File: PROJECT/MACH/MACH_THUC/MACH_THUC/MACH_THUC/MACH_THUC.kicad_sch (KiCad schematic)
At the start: 32 parts, among them Q1 2SB688, U1 LM7805_TO220

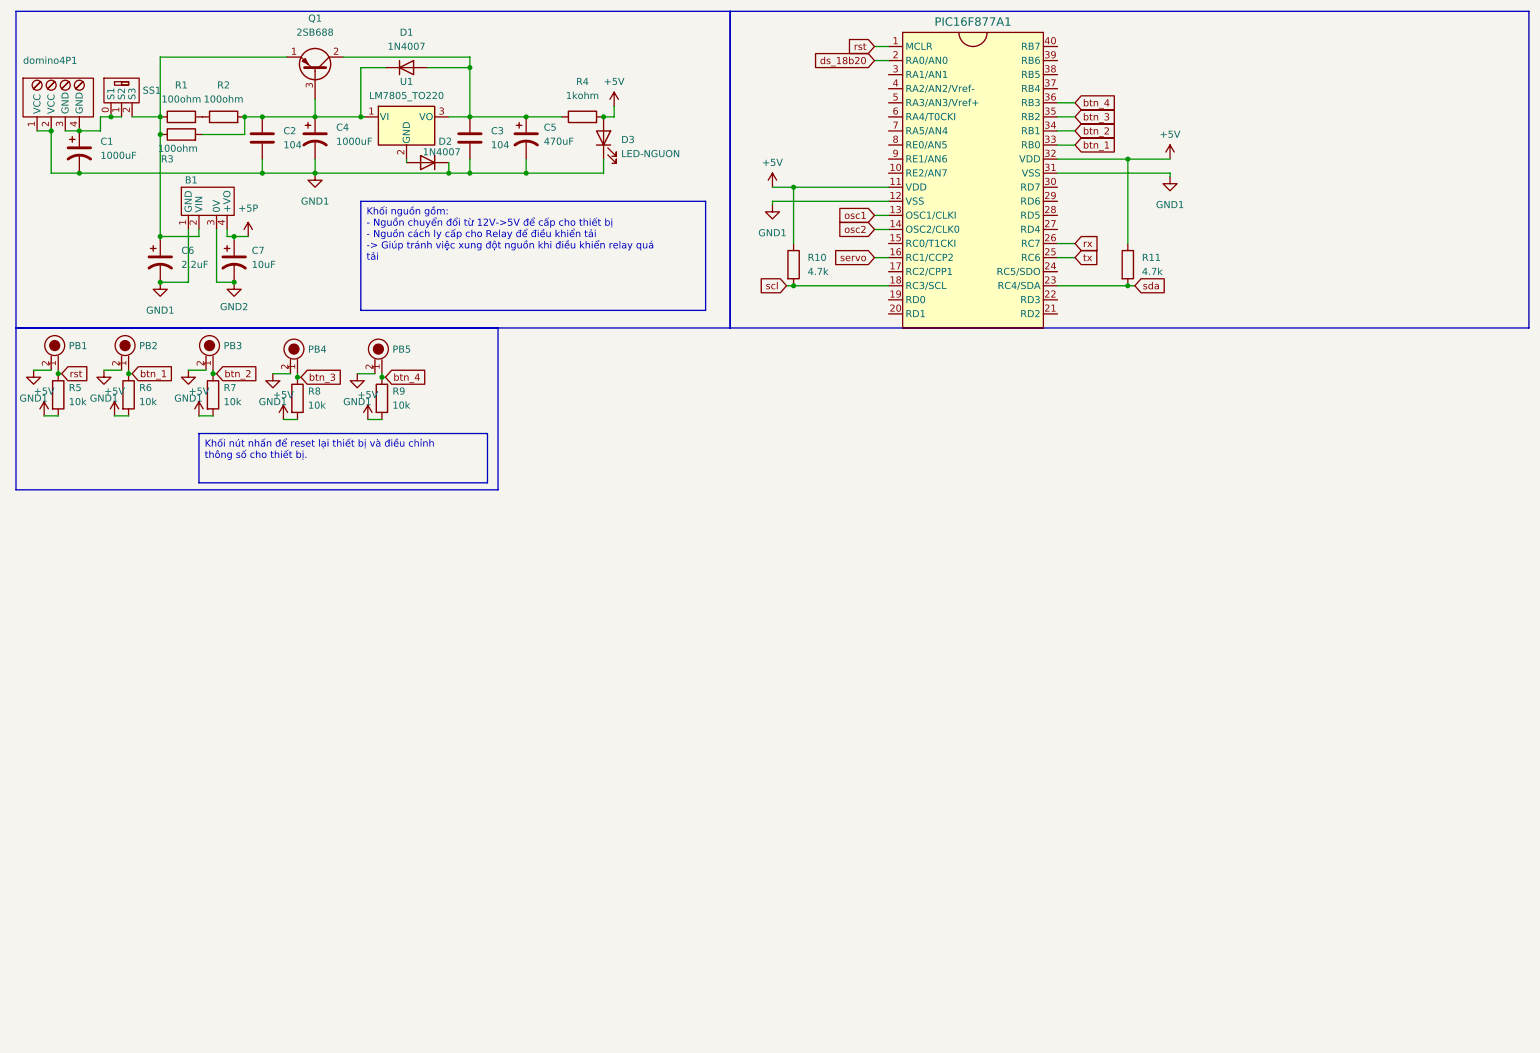
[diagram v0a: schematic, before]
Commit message: update code
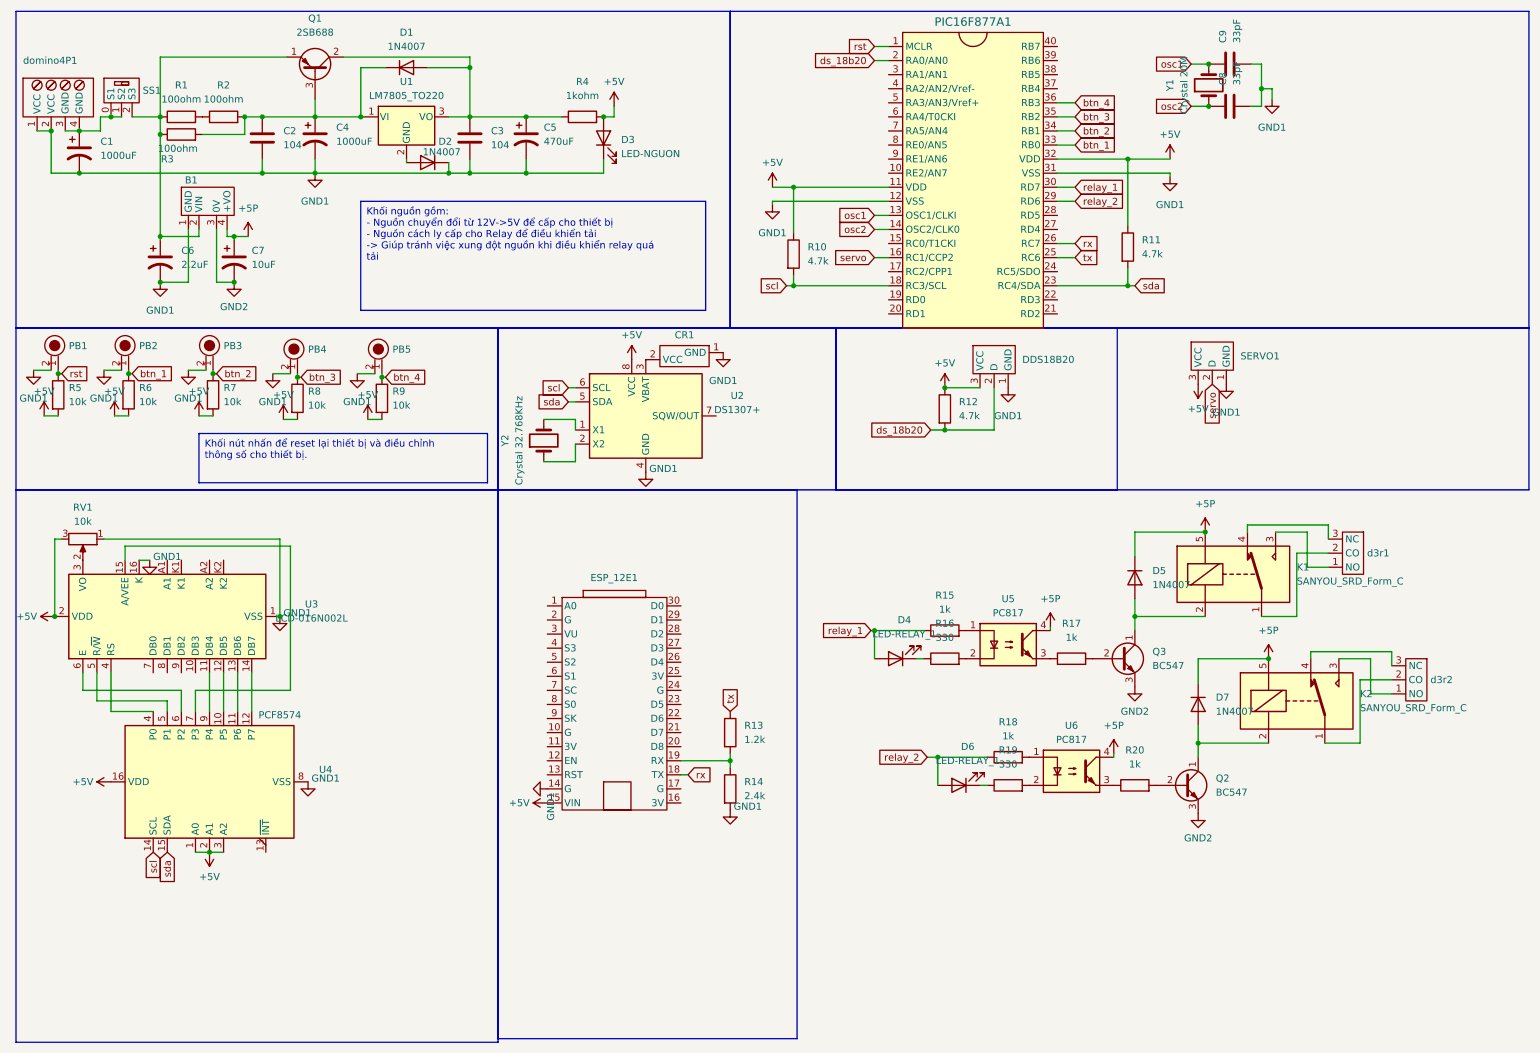
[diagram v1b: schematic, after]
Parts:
- added C8, C9: 33pF, library_thuan_footprint:CAP_104, symbol Device:C
- added CR1: ~, library_thuan_footprint:cr2032, symbol library_thuan:CR2032
- added D4, D6: LED-RELAY_1, library_thuan_footprint:LED_5MM, symbol Device:LED
- added D5, D7: 1N4007, library_thuan_footprint:1N4007, symbol Device:D
- added DDS18B20, SERVO1: ~, library_thuan_footprint:DOMINO_3, symbol library_thuan:domino_3pin
- added ESP_12E1: ~, library_thuan_footprint:ESP8266_12E, symbol library_thuan:ESP8266
- added K1, K2: SANYOU_SRD_Form_C, Relay_THT:Relay_SPDT_SANYOU_SRD_Series_Form_C, symbol Relay:SANYOU_SRD_Form_C
- added Q2, Q3: BC547, Package_TO_SOT_THT:TO-92_Inline, symbol Transistor_BJT:BC547
- added R12: 4.7k, library_thuan_footprint:RES_DEFAULT, symbol Device:R
- added R13: 1.2k, library_thuan_footprint:RES_DEFAULT, symbol Device:R
- added R14: 2.4k, library_thuan_footprint:RES_DEFAULT, symbol Device:R
- added R15, R17, R18, R20: 1k, library_thuan_footprint:RES_DEFAULT, symbol Device:R
- added R16, R19: 330, library_thuan_footprint:RES_DEFAULT, symbol Device:R
- added RV1: 10k, library_thuan_footprint:RM065-103, symbol Device:R_Potentiometer
- added U2: DS1307+, Package_DIP:DIP-8_W7.62mm, symbol Timer_RTC:DS1307+
- added U3: LCD-016N002L, Display:LCD-016N002L, symbol Display_Character:LCD-016N002L
- added U4: PCF8574, library_thuan_footprint:PCF8574, symbol Interface_Expansion:PCF8574
- added U5, U6: PC817, Package_DIP:DIP-4_W7.62mm, symbol Isolator:PC817
- added Y1: Crystal 20M, library_thuan_footprint:crytal_20M, symbol Device:Crystal
- added Y2: Crystal 32.768KHz, library_thuan_footprint:crytal_32.768KHz, symbol Device:Crystal
- added d3r1, d3r2: ~, library_thuan_footprint:DOMINO_3, symbol library_thuan:domino_3_relay
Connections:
- net +5P: now also D5.1 (K), D7.1 (K), K1.5, K2.5, U5.4, U6.4
- net +5V: now also DDS18B20.3 (VCC), ESP_12E1.15 (VIN), R12.1, RV1.3, SERVO1.3 (VCC), U2.8 (VCC), U3.2 (VDD), U4.1 (A0), U4.16 (VDD), U4.2 (A1), U4.3 (A2)
- net GND1: now also C8.2, C9.2, CR1.1 (GND), DDS18B20.1 (GND), ESP_12E1.14 (G), R14.2, RV1.1, SERVO1.1 (GND), U2.4 (GND), U3.1 (VSS), U3.16 (K), U4.8 (VSS)
- net GND2: now also Q2.3 (E), Q3.3 (E)
- net ds_18b20: now also DDS18B20.2 (D), R12.2
- net osc1: now also C9.1, Y1.2
- net osc2: now also C8.1, Y1.1
- net rx: now also ESP_12E1.18 (TX)
- net scl: now also U2.6 (SCL), U4.14 (SCL)
- net sda: now also U2.5 (SDA), U4.15 (SDA)
- net servo: now also SERVO1.2 (D)
- net tx: now also R13.1
- net relay_2: now reaches PIC16F877A1.29 (RD6)
- net relay_2: now also D6.2 (A), R18.1
- net relay_1: now reaches PIC16F877A1.30 (RD7)
- net relay_1: now also D4.2 (A), R15.1
- new net: D7.2 (A), K2.2, Q2.1 (C)
- new net: Q2.2 (B), R20.2
- new net: R15.2, U5.1
- new net: R16.2, U5.2
- new net: R17.1, U5.3
- new net: ESP_12E1.19 (RX), R13.2, R14.1
- new net: Q3.2 (B), R17.2
- new net: R18.2, U6.1
- new net: R19.2, U6.2
- new net: R20.1, U6.3
- new net: U2.1 (X1), Y2.2
- new net: U2.2 (X2), Y2.1
- new net: CR1.2 (VCC), U2.3 (VBAT)
- new net: K1.1, d3r1.2 (CO)
- new net: D5.2 (A), K1.2, Q3.1 (C)
- new net: K1.3, d3r1.1 (NO)
- new net: K1.4, d3r1.3 (NC)
- new net: K2.3, d3r2.1 (NO)
- new net: K2.1, d3r2.2 (CO)
- new net: K2.4, d3r2.3 (NC)
- new net: D6.1 (K), R19.1
- new net: U3.12 (DB5), U4.10 (P5)
- new net: U3.13 (DB6), U4.11 (P6)
- new net: U3.14 (DB7), U4.12 (P7)
- new net: U3.4 (RS), U4.4 (P0)
- new net: U3.5 (R/~{W}), U4.5 (P1)
- new net: U3.6 (E), U4.6 (P2)
- new net: U3.15 (A/VEE), U4.7 (P3)
- new net: U3.11 (DB4), U4.9 (P4)
- new net: D4.1 (K), R16.1
- new net: RV1.2, U3.3 (VO)
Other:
- moved on the sheet: R10, R11
